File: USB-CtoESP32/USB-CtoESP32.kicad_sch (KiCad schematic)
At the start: 24 parts, among them J1 USB_C_Receptacle_USB2.0_14P, J3 ICSP, SW1 RST, SW2 BOOT, U1 LM1117MP-3.3, U2 CH340G, Y1 12MHz

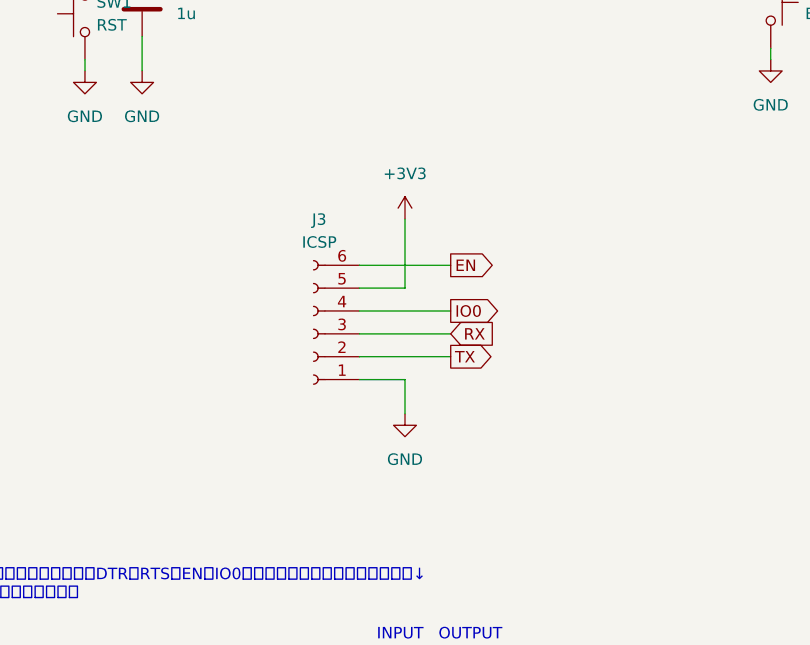
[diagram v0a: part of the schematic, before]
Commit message: Add files via upload
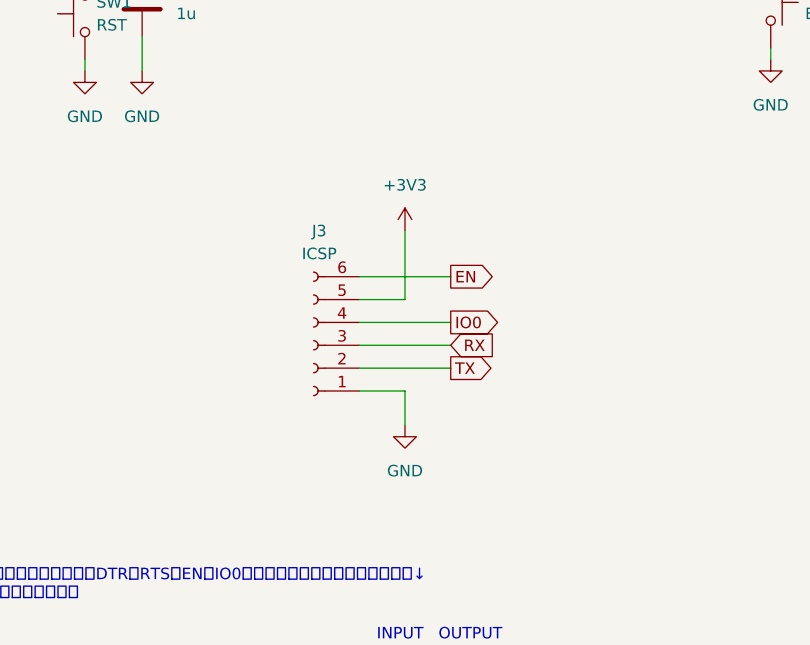
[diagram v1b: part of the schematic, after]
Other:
- moved on the sheet: J3
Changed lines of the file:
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@@
 	(wire
 		(pts
-			(xy 222.25 91.44) (xy 227.33 91.44)
-		)
-		(stroke
-			(width 0)
-			(type default)
-		)
-	)
-	(wire
-		(pts
-			(xy 222.25 83.82) (xy 232.41 83.82)
+			(xy 222.25 92.71) (xy 227.33 92.71)
+		)
+		(stroke
+			(width 0)
+			(type default)
+		)
+	)
+	(wire
+		(pts
+			(xy 222.25 85.09) (xy 232.41 85.09)
 		)
 		(stroke
@@
 	(wire
 		(pts
-			(xy 227.33 91.44) (xy 227.33 95.25)
+			(xy 227.33 92.71) (xy 227.33 96.52)
 		)
 		(stroke
@@
 	(wire
 		(pts
-			(xy 222.25 81.28) (xy 227.33 81.28)
+			(xy 222.25 82.55) (xy 227.33 82.55)
 		)
 		(stroke
@@
 	(wire
 		(pts
-			(xy 222.25 86.36) (xy 232.41 86.36)
+			(xy 222.25 87.63) (xy 232.41 87.63)
 		)
 		(stroke
@@
 	(wire
 		(pts
-			(xy 222.25 78.74) (xy 232.41 78.74)
+			(xy 222.25 80.01) (xy 232.41 80.01)
 		)
 		(stroke
@@
 	(wire
 		(pts
-			(xy 227.33 81.28) (xy 227.33 73.66)
+			(xy 227.33 82.55) (xy 227.33 74.93)
 		)
 		(stroke
@@
 	(wire
 		(pts
-			(xy 222.25 88.9) (xy 232.41 88.9)
+			(xy 222.25 90.17) (xy 232.41 90.17)
 		)
 		(stroke
@@
 	(global_label "TX"
 		(shape output)
-		(at 232.41 88.9 0)
+		(at 232.41 90.17 0)
 		(fields_autoplaced yes)
 		(effects
@@
 		)
 		(property "Intersheetrefs" "${INTERSHEET_REFS}"
-			(at 237.5723 88.9 0)
+			(at 237.5723 90.17 0)
 			(effects
 				(font
@@
 	(global_label "EN"
 		(shape output)
-		(at 232.41 78.74 0)
+		(at 232.41 80.01 0)
 		(fields_autoplaced yes)
 		(effects
@@
 		)
 		(property "Intersheetrefs" "${INTERSHEET_REFS}"
-			(at 237.8747 78.74 0)
+			(at 237.8747 80.01 0)
 			(effects
 				(font
@@
 	(global_label "IO0"
 		(shape output)
-		(at 232.41 83.82 0)
+		(at 232.41 85.09 0)
 		(fields_autoplaced yes)
 		(effects
@@
 		)
 		(property "Intersheetrefs" "${INTERSHEET_REFS}"
-			(at 238.54 83.82 0)
+			(at 238.54 85.09 0)
 			(effects
 				(font
@@
 	(global_label "RX"
 		(shape input)
-		(at 232.41 86.36 0)
+		(at 232.41 87.63 0)
 		(fields_autoplaced yes)
 		(effects
@@
 		)
 		(property "Intersheetrefs" "${INTERSHEET_REFS}"
-			(at 237.8747 86.36 0)
+			(at 237.8747 87.63 0)
 			(effects
 				(font
@@
 	(symbol
 		(lib_id "power:+5V")
-		(at 227.33 73.66 0)
+		(at 227.33 74.93 0)
 		(unit 1)
 		(exclude_from_sim no)
@@
 		(fields_autoplaced yes)
 		(property "Reference" "#PWR014"
-			(at 227.33 77.47 0)
+			(at 227.33 78.74 0)
 			(effects
 				(font
@@
 		)
 		(property "Value" "+3V3"
-			(at 227.33 68.58 0)
+			(at 227.33 69.85 0)
 			(effects
 				(font
@@
 		)
 		(property "Footprint" ""
-			(at 227.33 73.66 0)
+			(at 227.33 74.93 0)
 			(effects
 				(font
@@
 		)
 		(property "Datasheet" ""
-			(at 227.33 73.66 0)
+			(at 227.33 74.93 0)
 			(effects
 				(font
@@
 		)
 		(property "Description" "Power symbol creates a global label with name \"+5V\""
-			(at 227.33 73.66 0)
+			(at 227.33 74.93 0)
 			(effects
 				(font
@@
 	(symbol
 		(lib_id "Connector:Conn_01x06_Socket")
-		(at 217.17 86.36 180)
+		(at 217.17 87.63 180)
 		(unit 1)
 		(exclude_from_sim no)
@@
 		(fields_autoplaced yes)
 		(property "Reference" "J3"
-			(at 217.805 73.66 0)
+			(at 217.805 74.93 0)
 			(effects
 				(font
@@
 		)
 		(property "Value" "ICSP"
-			(at 217.805 76.2 0)
+			(at 217.805 77.47 0)
 			(effects
 				(font
@@
 		)
 		(property "Footprint" "Connector_PinHeader_2.54mm:PinHeader_2x03_P2.54mm_Horizontal"
-			(at 217.17 86.36 0)
+			(at 217.17 87.63 0)
 			(effects
 				(font
@@
 		)
 		(property "Datasheet" "~"
-			(at 217.17 86.36 0)
+			(at 217.17 87.63 0)
 			(effects
 				(font
@@
 		)
 		(property "Description" "Generic connector, single row, 01x06, script generated"
-			(at 217.17 86.36 0)
+			(at 217.17 87.63 0)
 			(effects
 				(font
@@
 	(symbol
 		(lib_id "power:GND")
-		(at 227.33 95.25 0)
+		(at 227.33 96.52 0)
 		(unit 1)
 		(exclude_from_sim no)
@@
 		(fields_autoplaced yes)
 		(property "Reference" "#PWR015"
+			(at 227.33 102.87 0)
+			(effects
+				(font
+					(size 1.27 1.27)
+				)
+				(hide yes)
+			)
+		)
+		(property "Value" "GND"
 			(at 227.33 101.6 0)
 			(effects
@@
 					(size 1.27 1.27)
 				)
-				(hide yes)
-			)
-		)
-		(property "Value" "GND"
-			(at 227.33 100.33 0)
-			(effects
-				(font
-					(size 1.27 1.27)
-				)
 			)
 		)
 		(property "Footprint" ""
-			(at 227.33 95.25 0)
+			(at 227.33 96.52 0)
 			(effects
 				(font
@@
 		)
 		(property "Datasheet" ""
-			(at 227.33 95.25 0)
+			(at 227.33 96.52 0)
 			(effects
 				(font
@@
 		)
 		(property "Description" "Power symbol creates a global label with name \"GND\" , ground"
-			(at 227.33 95.25 0)
-			(effects
-				(font
+			(at 227.33 96.52 0)
+			(effects
+				(font
